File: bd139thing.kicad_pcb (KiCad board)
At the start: 2 copper layers, 75 x 75 mm, 26 parts, among them J1 Audio-Jack-3, J2 Jack-DC, Q1 PN2222, Q2 BD13916, Q3 BD13916, Q4 PN2222, Q5 BD13916, Q6 BD13916

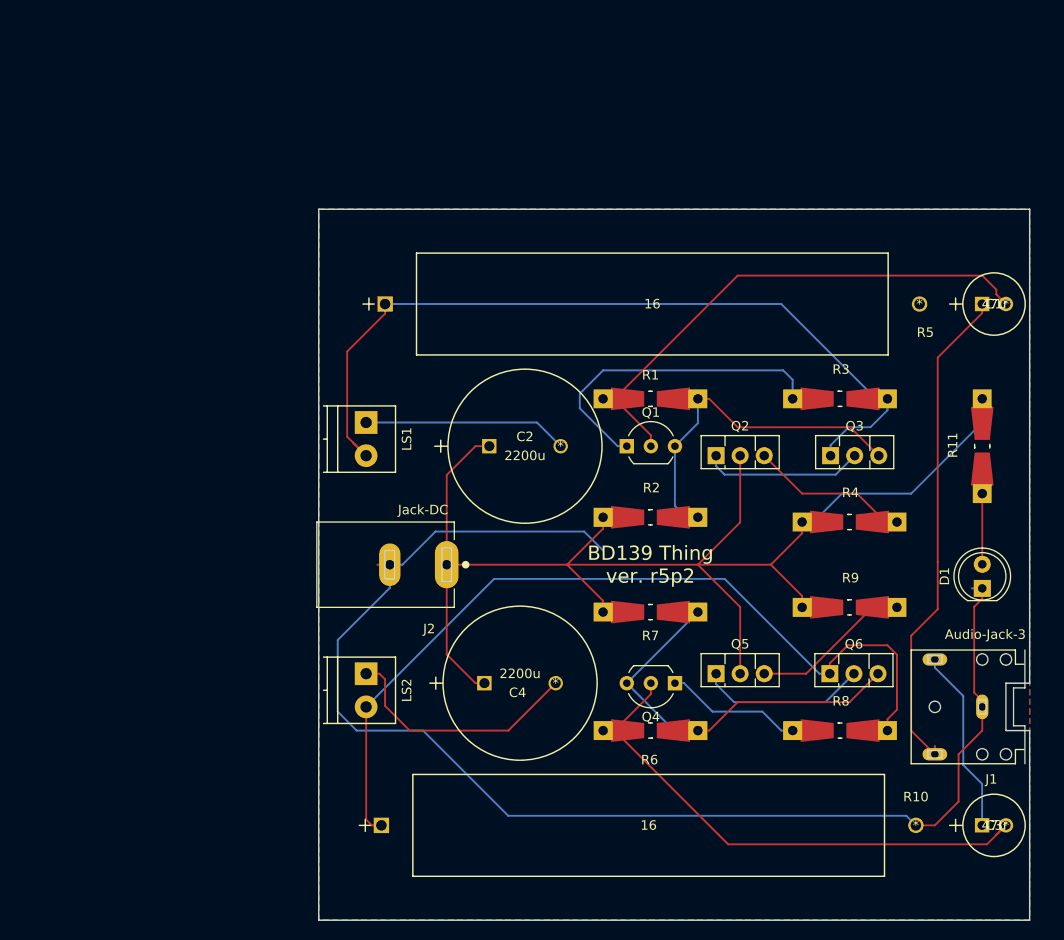
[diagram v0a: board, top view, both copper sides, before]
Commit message: 6 ok
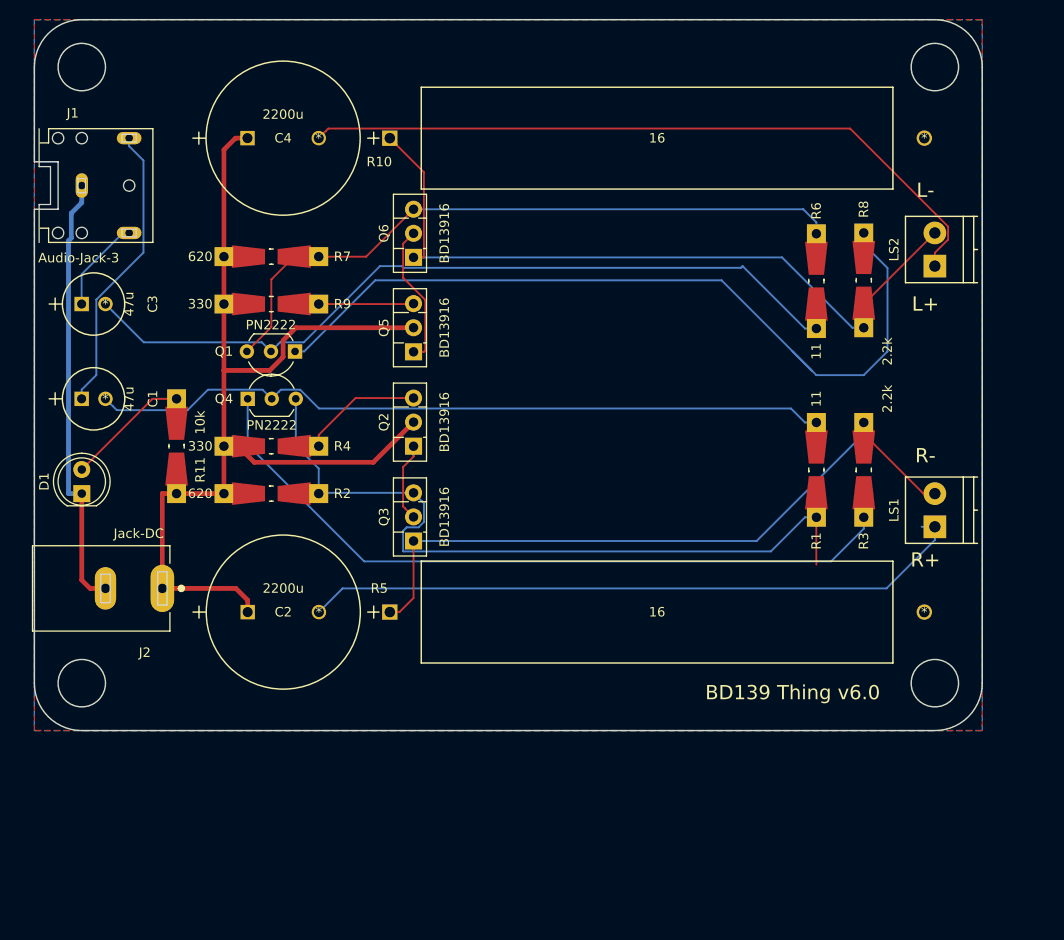
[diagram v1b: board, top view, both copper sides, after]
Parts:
- moved C3 109.8 mm to (7.50, 30.0)
- moved J1 109.8 mm to (5.00, 17.5), turned to 0 degrees
- moved C1 95.5 mm to (7.50, 40.0)
- moved D1 95.5 mm to (5.00, 50.0)
- moved R11 85.0 mm to (15.0, 45.0), turned to 270 degrees
- moved LS2 73.8 mm to (95.0, 26.0), turned to 90 degrees
- moved R10 72.5 mm to (93.9, 12.5)
- moved R9 68.9 mm to (25.0, 30.0)
- moved C4 62.7 mm to (30.0, 12.5)
- moved Q6 62.1 mm to (40.0, 25.1), turned to 90 degrees
- moved R4 61.5 mm to (25.0, 45.0)
- moved LS1 61.0 mm to (95.0, 53.5), turned to 90 degrees
- moved R7 54.8 mm to (25.0, 25.0)
- moved Q4 53.2 mm to (27.5, 35.0)
- moved R6 50.5 mm to (82.5, 27.6), turned to 270 degrees
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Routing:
- net GND: track 141.4 -> 46.5 mm
- net Net-(Q4-Pad1): track 17.1 -> 89.8 mm
- net Net-(C4-Pad2): track 26.2 -> 75.9 mm
- net Net-(C2-Pad2): track 21.6 -> 70.9 mm
- net Net-(Q1-Pad1): track 36.6 -> 80.2 mm
- net Net-(Q1-Pad3): track 41.9 -> 84.6 mm
- net Net-(C3-Pad2): track 56.3 -> 86.3 mm
- net Net-(Q4-Pad3): track 46.8 -> 73.6 mm
- net +12V: track 151.2 -> 124.8 mm
- net Net-(C1-Pad1): track 54.3 -> 30.8 mm
- net Net-(C1-Pad2): track 58.6 -> 81.2 mm
- net Net-(LS1-Pad2): track 90.5 -> 76.4 mm
- net Net-(LS2-Pad2): track 92.8 -> 81.4 mm
- net Net-(C3-Pad1): track 19.6 -> 9.96 mm
- net Net-(Q2-Pad1): track 16.9 -> 9.47 mm
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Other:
- board size 75 x 75 mm -> 100 x 75 mm
- net class Power added: clearance 0.25, trace_width 0.5, via_dia 0.75, via_drill 0.7
- board text added: "BD139 Thing v6.0"
- board text added: "L+"
- board text added: "L-"
- board text added: "R+"
- board text added: "R-"
- board text removed: "BD139 Thing ver. r5p2"
